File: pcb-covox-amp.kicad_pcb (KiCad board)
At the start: 2 copper layers, 78 x 56 mm, 45 parts, among them J1 DB25, P1 USB, U1 LM386, X1 Amp, X2 Raw

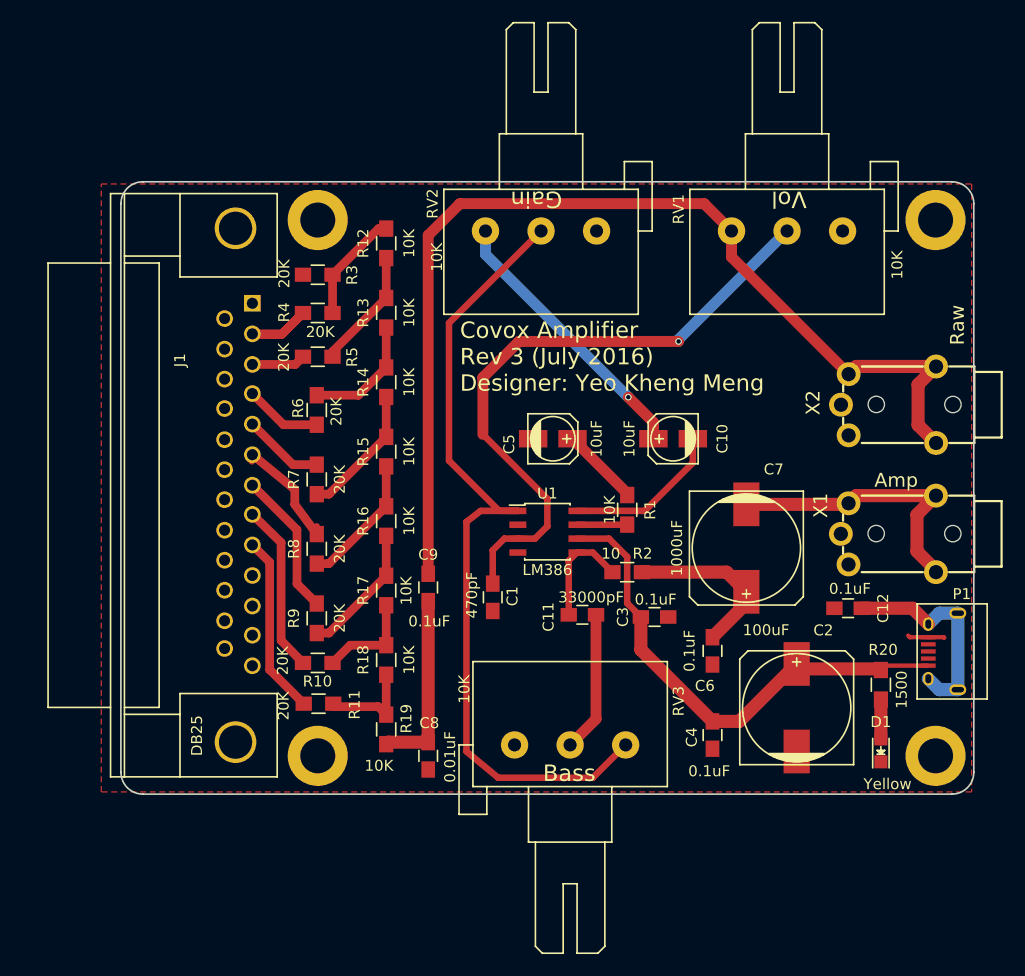
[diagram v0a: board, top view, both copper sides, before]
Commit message: updated modded version
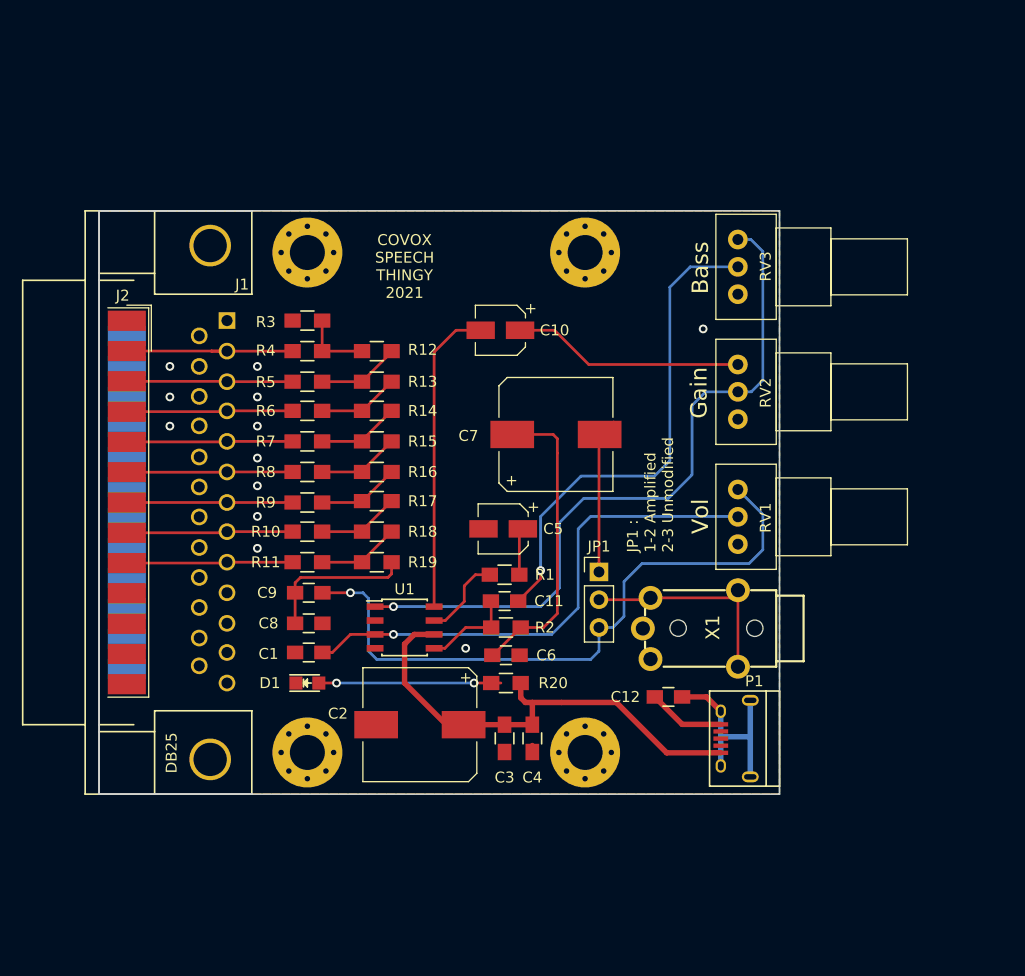
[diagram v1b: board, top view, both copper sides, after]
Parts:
- removed X2: Raw, mj2135:mj-2135-MJ-2135
- added J2: DB25, Sebs:DSUB-25_Male_EdgeMount_P2.77mm, F.Cu at (102.5, 115.3)
- added JP1: Jumper_3_Open, Pin_Headers:Pin_Header_Straight_1x03_Pitch2.54mm, F.Cu at (145.7, 121.7)
- C10, C5: footprint Capacitors_SMD:c_elec_4x5.3 -> Capacitors_SMD:CP_Elec_4x5.3
- C2, C7: footprint Capacitors_SMD:c_elec_10x10.5 -> Capacitors_SMD:CP_Elec_10x10.5
- MH1, MH2, MH3, MH4: footprint Mounting_Holes:MountingHole_3.2mm_M3_ISO14580_Pad -> Mounting_Holes:MountingHole_3.2mm_M3_Pad_Via
- RV1, RV2, RV3: footprint Potentiometers:Potentiometer_Alps-RK163-single_15mm -> Potentiometers:Potentiometer_Alps_RK09Y_Vertical
- X1: footprint mj2135:mj-2135-MJ-2135 -> Sebs:mj-2135-MJ-2135
- moved D1 52.8 mm to (119.0, 131.8), turned to 0 degrees
- moved RV3 46.0 mm to (158.4, 96.3), turned to 0 degrees
- moved C2 34.5 mm to (129.3, 135.7), turned to 180 degrees
- moved R20 34.3 mm to (137.2, 131.8), turned to 180 degrees
- moved MH1 32.2 mm to (144.4, 92.5)
- moved MH2 32.1 mm to (144.4, 138.2)
- moved RV1 30.2 mm to (158.4, 119.1), turned to 0 degrees
- moved RV2 21.5 mm to (158.4, 107.7), turned to 0 degrees
- moved P1 20.6 mm to (158.4, 136.9)
- moved C7 20.3 mm to (141.8, 109.1), turned to 0 degrees
- moved X1 20.1 mm to (155.9, 126.8)
- moved C6 18.9 mm to (137.2, 129.3), turned to 0 degrees
- moved C10 18.7 mm to (136.7, 99.6)
- moved C12 18.3 mm to (152.1, 133.1)
- moved C3 17.6 mm to (137.1, 136.9), turned to 270 degrees
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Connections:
- J1 pad 1: (no net) -> Net-(J1-Pad1)
- J1 pad 10: (no net) -> Net-(J1-Pad10)
- J1 pad 11: (no net) -> Net-(J1-Pad11)
- J1 pad 12: (no net) -> Net-(J1-Pad12)
- J1 pad 13: (no net) -> Net-(J1-Pad13)
- J1 pad 14: (no net) -> Net-(J1-Pad14)
- J1 pad 15: (no net) -> Net-(J1-Pad15)
- J1 pad 16: (no net) -> Net-(J1-Pad16)
- J1 pad 17: (no net) -> Net-(J1-Pad17)
- MH1 pad 1: (no net) -> GND
- MH2 pad 1: (no net) -> GND
- MH3 pad 1: (no net) -> GND
- MH4 pad 1: (no net) -> GND
- P1 pad 2: (no net) -> Net-(P1-Pad2)
- P1 pad 3: (no net) -> Net-(P1-Pad3)
- P1 pad 4: (no net) -> Net-(P1-Pad4)
- RV2 pad 1: (no net) -> Net-(RV2-Pad1)
- RV3 pad 1: (no net) -> Net-(RV3-Pad1)
- X1 pad P$1: (no net) -> Net-(X1-PadP$1)
- X1 pad P$3: Amp-Audio -> Net-(JP1-Pad2)
- X1 pad P$4: Amp-Audio -> Net-(JP1-Pad2)
- X1 pad P$5: Amp-Audio -> Net-(JP1-Pad2)
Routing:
- net Source-Audio: track 95.1 -> 59.4 mm, vias 0 -> 1
- net Net-(C11-Pad2): track 12.9 -> 45.4 mm, vias 0 -> 1
- net Net-(JP1-Pad2): track 0.00 -> 20.1 mm
- net Gain8: track 14.6 -> 28.4 mm
- net Net-(D1-Pad2): track 3.60 -> 16.7 mm, vias 0 -> 2
- net Net-(C6-Pad1): track 15.7 -> 27.9 mm
- net Amp-Audio: track 26.1 -> 14.3 mm
- net Input+: track 58.7 -> 47.4 mm
- net Data1: track 4.92 -> 15.2 mm
- net Gain1: track 75.4 -> 65.8 mm, vias 0 -> 1
- net Data2: track 7.22 -> 15.2 mm
- net Data3: track 7.43 -> 15.2 mm
- net Data0: track 10.9 -> 16.6 mm
- net Net-(R16-Pad1): track 12.2 -> 7.51 mm
- net GND: track 3.38 -> 8.01 mm, vias 0 -> 12
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- added copper zone on B.Cu, net GND
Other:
- board size 78 x 56 mm -> 62.2 x 53.3 mm
- net class Default: via_dia 0.6 -> 0.8; via_drill 0.4 -> 0.45
- net class Micro-USB: via_drill 0.4 -> 0.45
- rule via_min_drill: 0.3 -> 0.45
- rule via_min_size: 0.4 -> 0.45
- board text added: "Based on design by Yeo Kheng Meng (https://github.com/yeokm1/pcb-covox-amp)"
- board text added: "COVOX SPEECH THINGY 2021"
- board text added: "JP1 : 1-2 Amplified 2-3 Unmodified"
- board text added: "https://pcb.hegars.com/?sku=covox2021?sn="
- board text removed: "Covox Amplifier Rev 3 (July 2016) Designer: Yeo Kheng Meng"
